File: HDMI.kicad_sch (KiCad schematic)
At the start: 10 parts, among them IC6 TPS2553QDBVRQ1, J9 HDMI_E

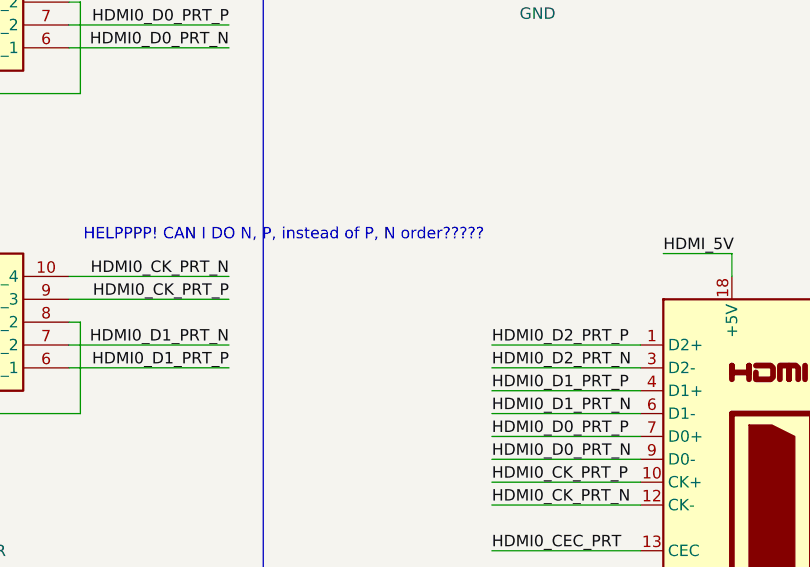
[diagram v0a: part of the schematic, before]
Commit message: small notes
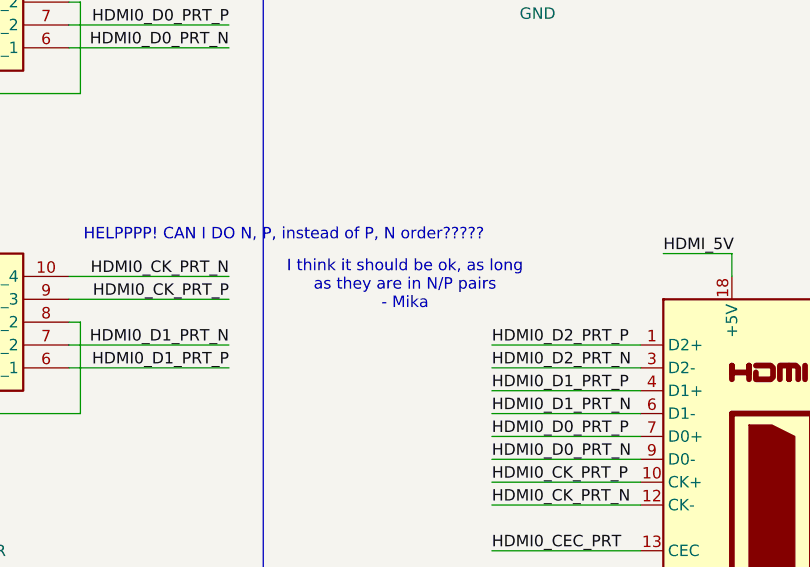
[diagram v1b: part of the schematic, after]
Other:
- note added: "I think it should be ok, as long as they are in N/P pairs - Mika"
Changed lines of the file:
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@@
+		)
+	)
+	(text "I think it should be ok, as long\nas they are in N/P pairs\n- Mika\n"
+		(exclude_from_sim no)
+		(at 213.868 98.806 0)
+		(effects
+			(font
+				(size 1.27 1.27)
+			)
 		)
 	)
